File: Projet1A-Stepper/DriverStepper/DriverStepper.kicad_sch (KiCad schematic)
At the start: 26 parts, among them IC1 AS5600-ASOT, IC2 TMC2225-SA, J1 Conn_01x04_Pin, J2 173010542, U1 STM32F446RETx, U2 AZ1117IH-3.3TRG1

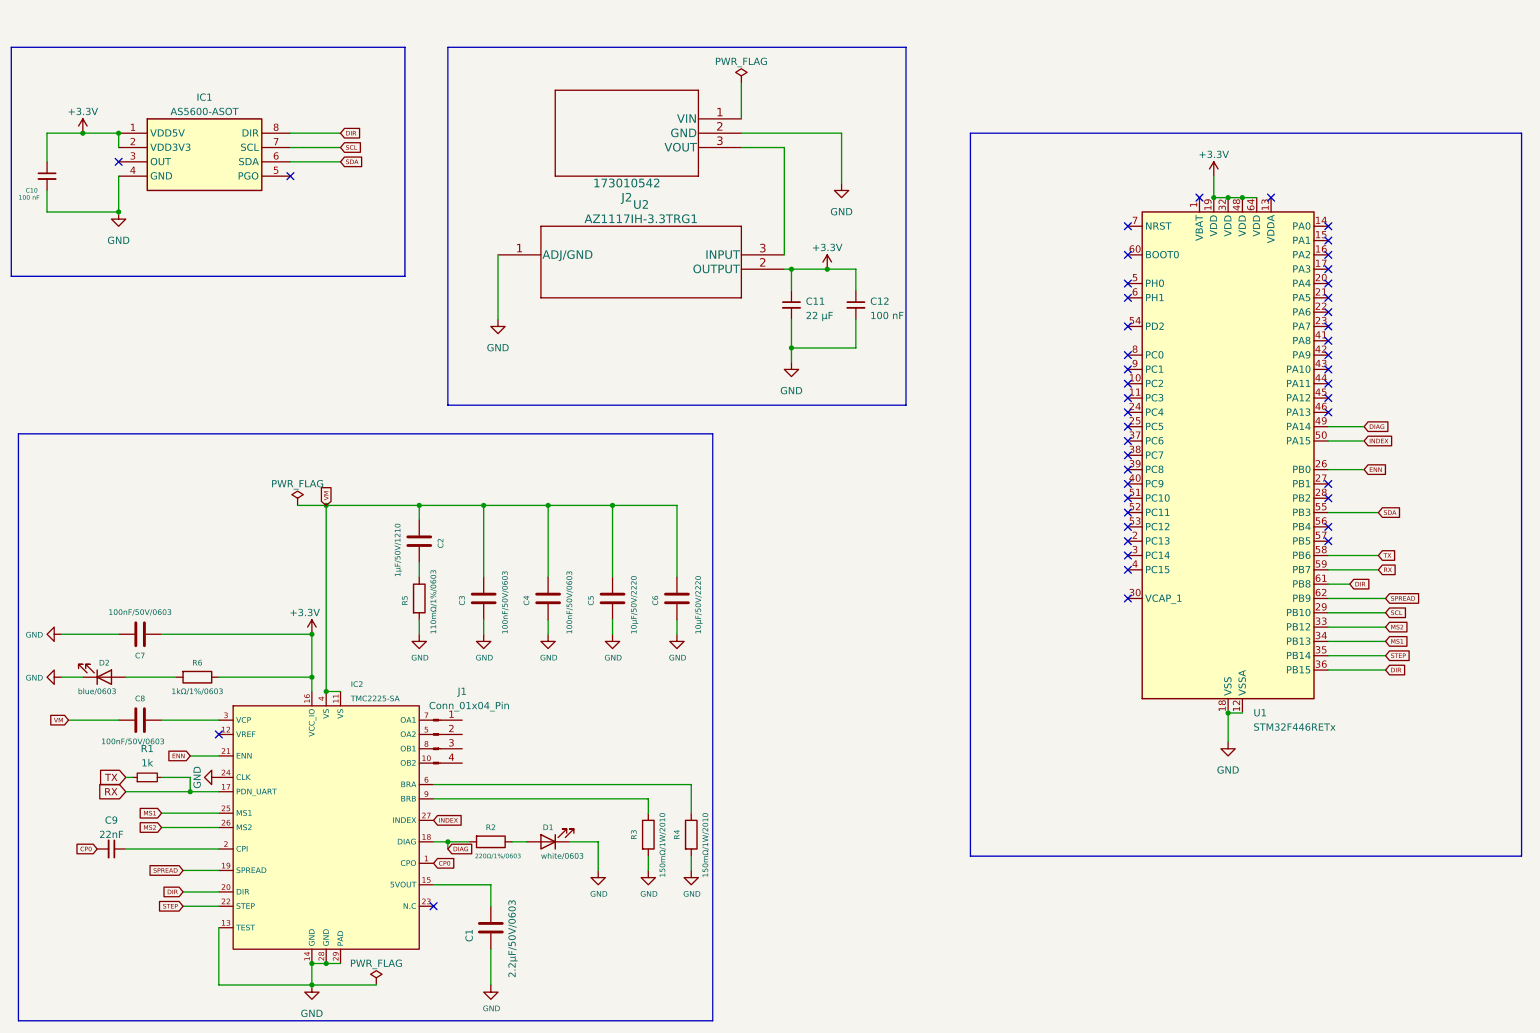
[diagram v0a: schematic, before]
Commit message: Add files via upload
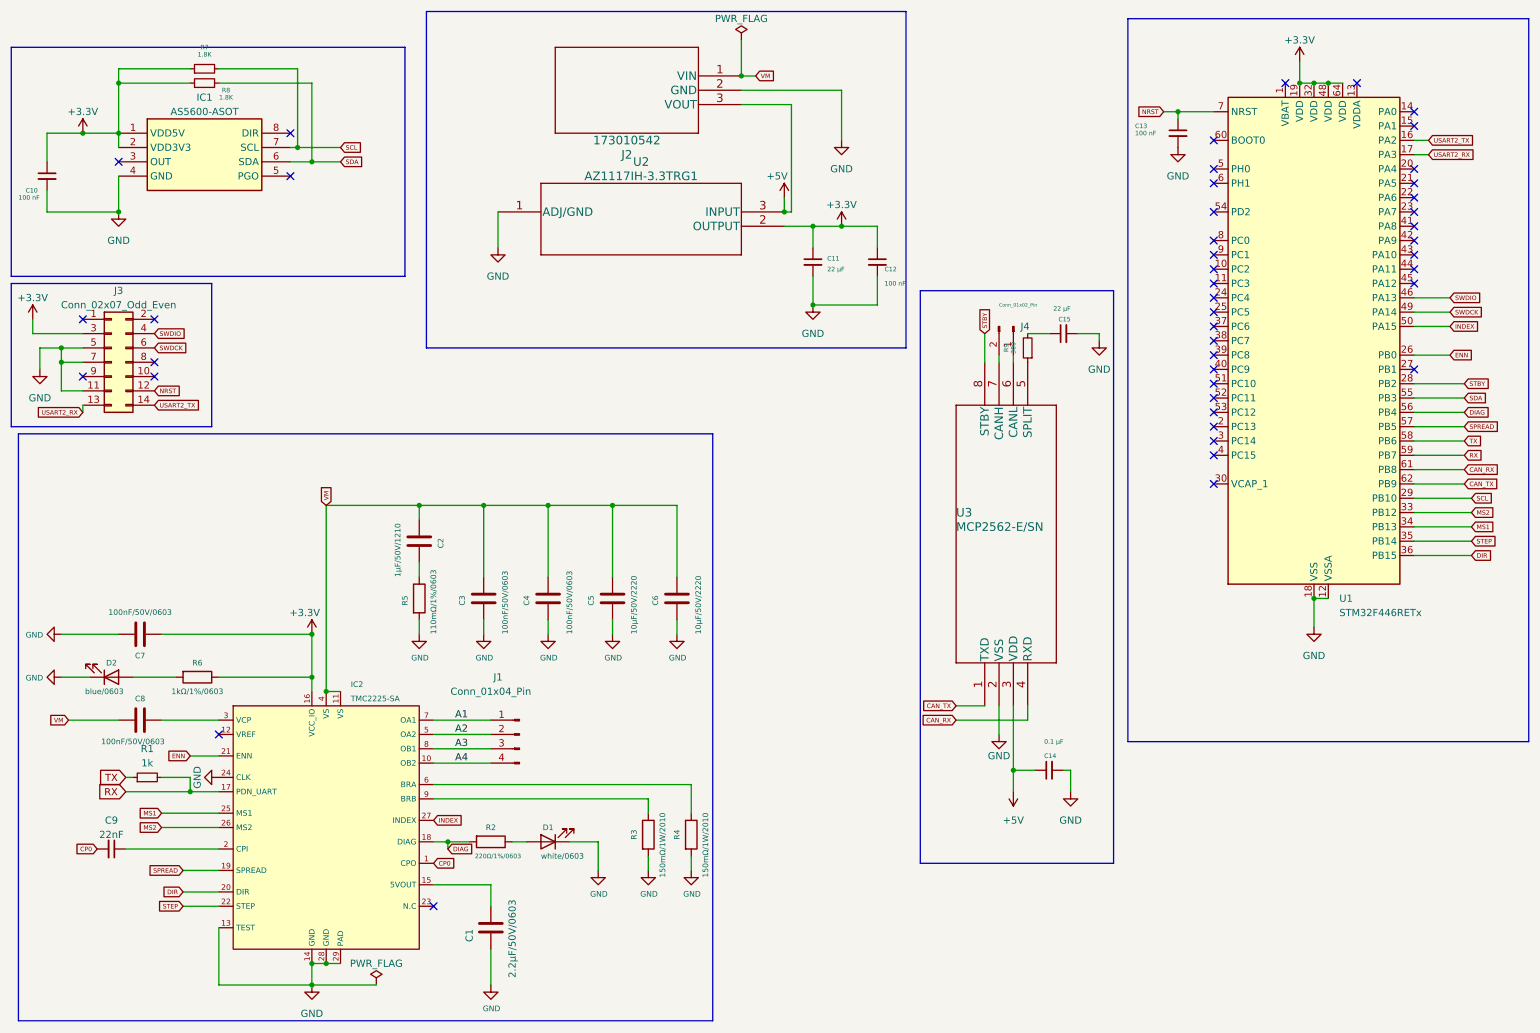
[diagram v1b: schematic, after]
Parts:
- added C13: 100 nF, symbol Device:C_Small
- added C14: 0.1 µF, symbol Device:C_Small
- added C15: 22 µF, symbol Device:C_Small
- added J3: Conn_02x07_Odd_Even, symbol Connector_Generic:Conn_02x07_Odd_Even
- added J4: Conn_01x02_Pin, symbol Connector:Conn_01x02_Pin
- added R7, R8: 1.8K, symbol Device:R_Small
- added R9: 300, symbol Device:R_Small
- added U3: MCP2562-E/SN, SOIC8-N_MC_MCH, symbol MCP2562-E/SN:MCP2562-E/SN
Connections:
- net +3.3V: now also J3.3 (Pin_3), R7.1, R8.1
- net DIAG: now also U1.56 (PB4); no longer U1.49 (PA14)
- net DIR: no longer IC1.8 (DIR), U1.61 (PB8)
- net GND: now also C13.2, C14.2, C15.2, J3.11 (Pin_11), J3.5 (Pin_5), J3.7 (Pin_7), U3.2 (VSS)
- net SCL: now also R7.2
- net SDA: now also R8.2
- net SPREAD: now also U1.57 (PB5); no longer U1.62 (PB9)
- net VM: now also J2.1 (VIN)
- net +5V: now reaches J2.3 (VOUT), U2.3 (INPUT)
- net +5V: now also C14.1, U3.3 (VDD)
- net A4: now reaches IC2.10 (OB2)
- net A4: now also J1.4 (Pin_4)
- net A2: now reaches IC2.5 (OA2)
- net A2: now also J1.2 (Pin_2)
- net A1: now reaches IC2.7 (OA1)
- net A1: now also J1.1 (Pin_1)
- net A3: now reaches IC2.8 (OB1)
- net A3: now also J1.3 (Pin_3)
- net USART2_TX: now reaches U1.16 (PA2)
- net USART2_TX: now also J3.14 (Pin_14)
- net USART2_RX: now reaches U1.17 (PA3)
- net USART2_RX: now also J3.13 (Pin_13)
- net STBY: now reaches U1.28 (PB2)
- net STBY: now also U3.8 (STBY)
- net SWDIO: now reaches U1.46 (PA13)
- net SWDIO: now also J3.4 (Pin_4)
- net NRST: now reaches U1.7 (NRST)
- net NRST: now also C13.1, J3.12 (Pin_12)
- new net: R9.1, U3.5 (SPLIT)
- new net: C15.1, R9.2
- new net: J4.1 (Pin_1), U3.6 (CANL)
- new net: J4.2 (Pin_2), U3.7 (CANH)
- new net CAN_RX: U1.61 (PB8), U3.4 (RXD)
- new net CAN_TX: U1.62 (PB9), U3.1 (TXD)
- new net SWDCK: J3.6 (Pin_6), U1.49 (PA14)
- no-connect marks 46 -> 45
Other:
- moved on the sheet: C11, C12, D2, J1, J2, U1, U2

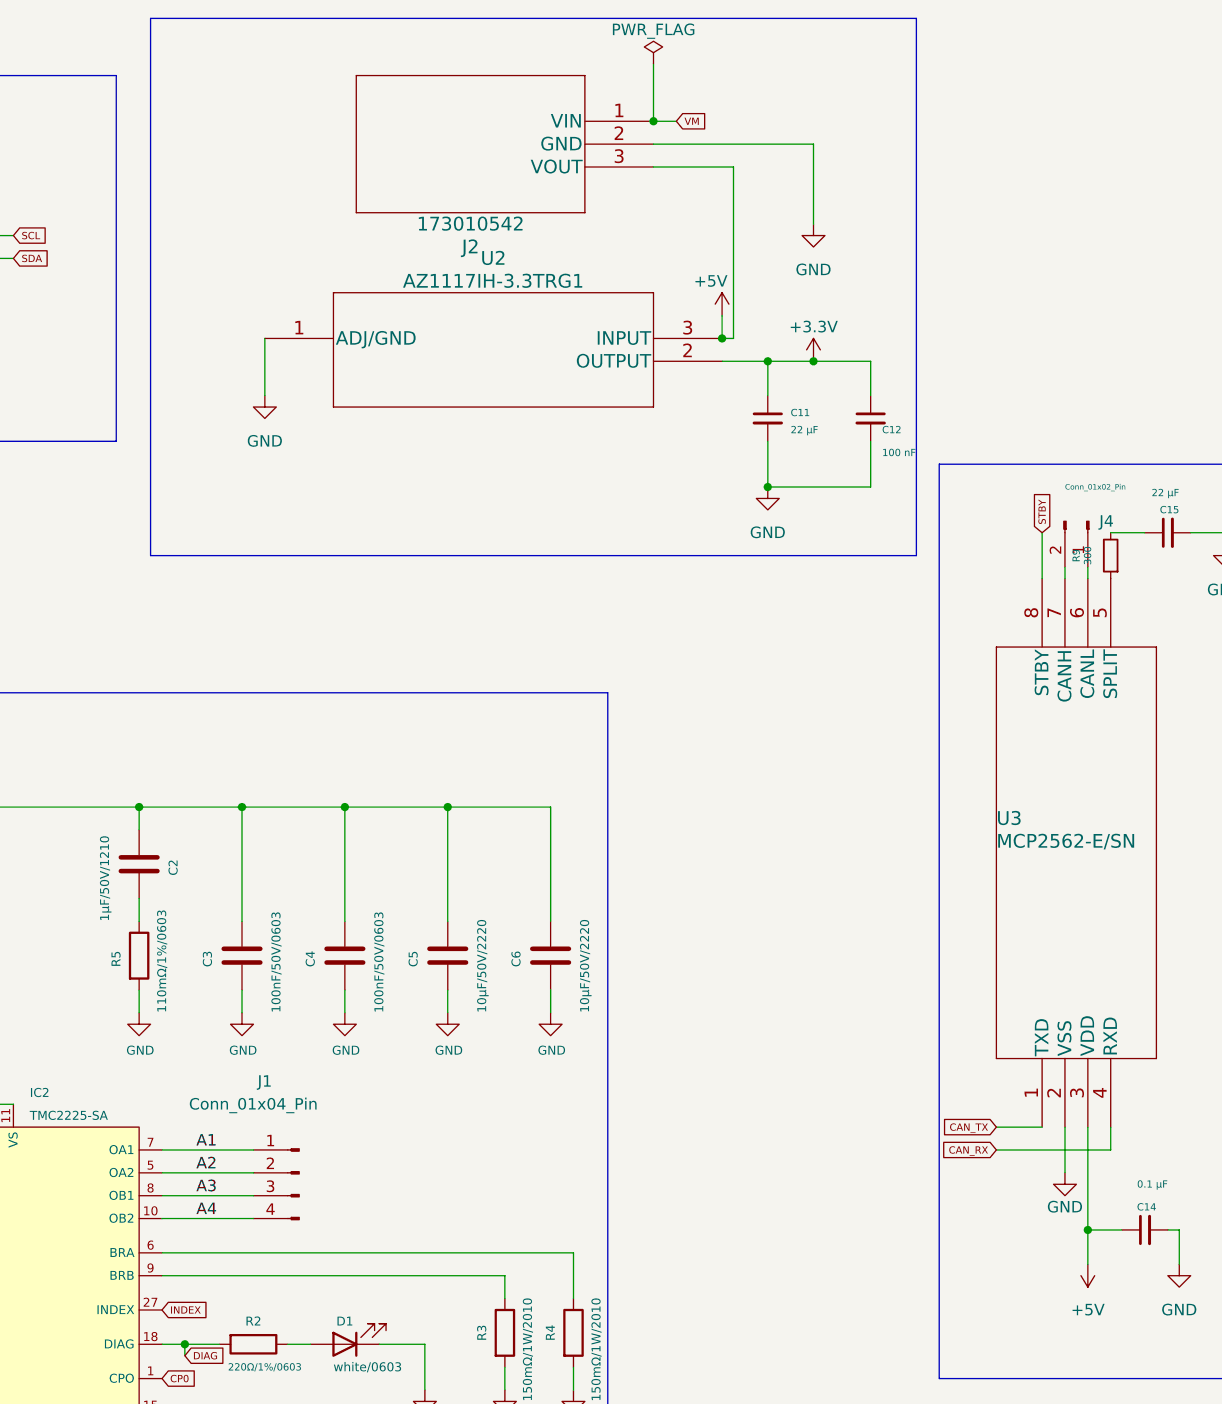
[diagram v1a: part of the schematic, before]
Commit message: Add files via upload
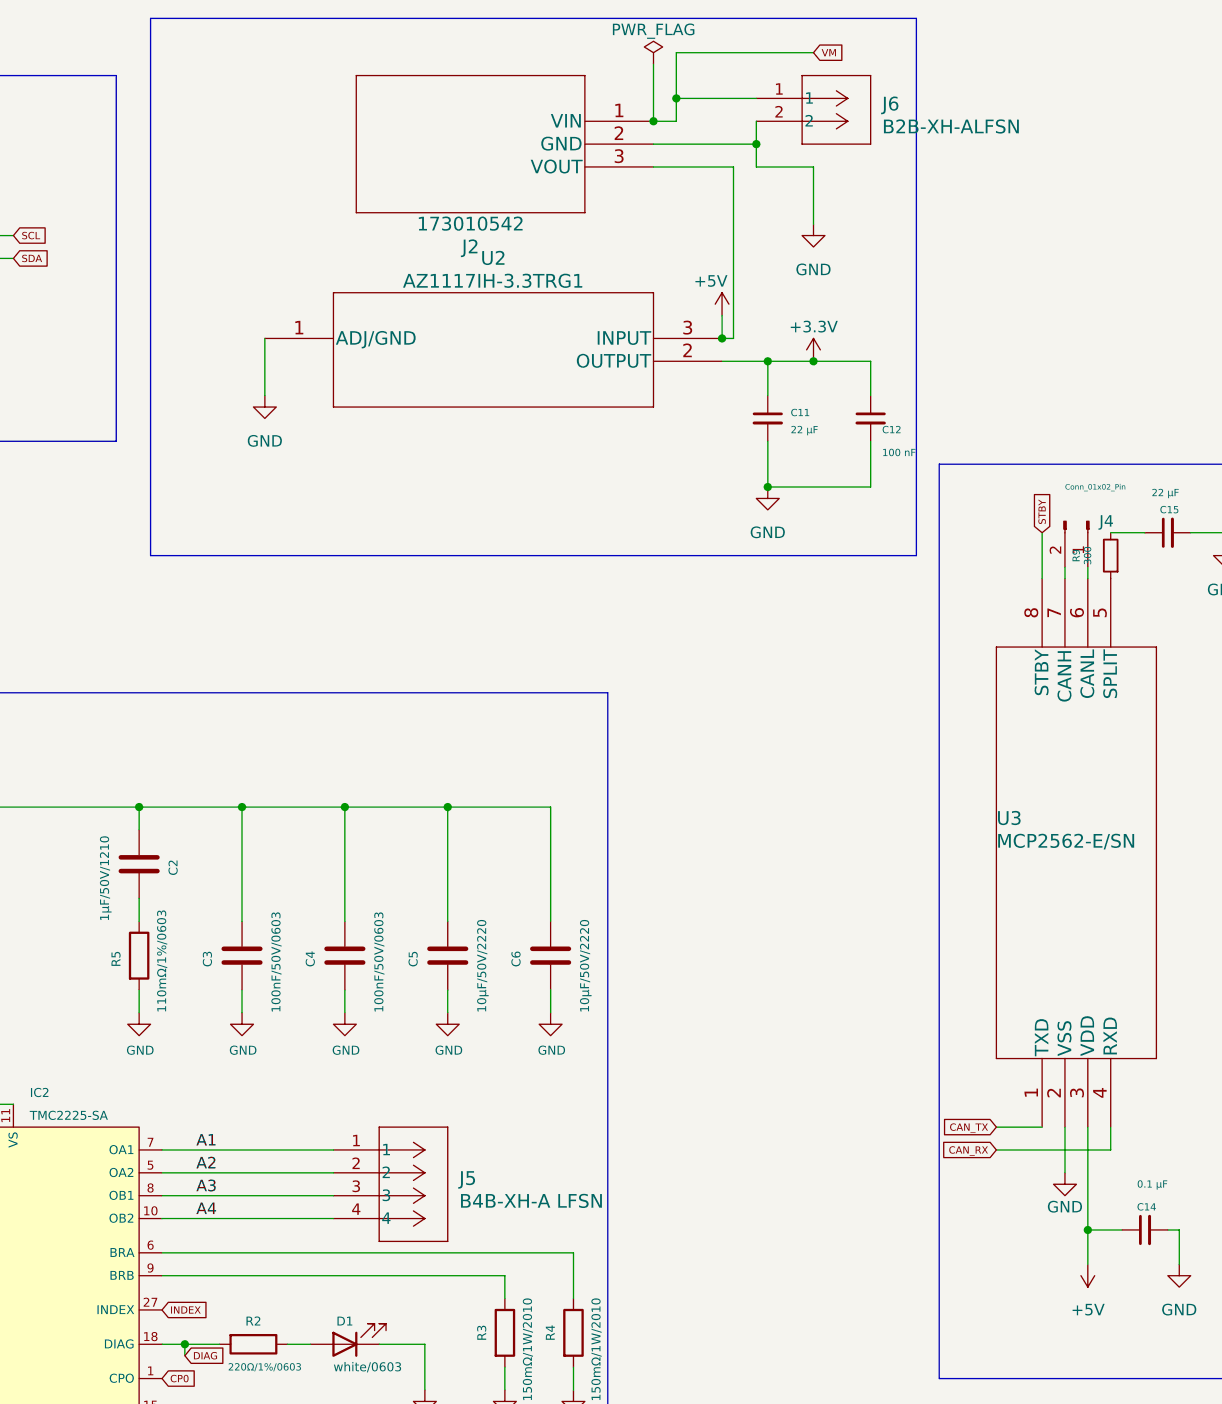
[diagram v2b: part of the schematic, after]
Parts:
- removed J1: Conn_01x04_Pin, symbol Connector:Conn_01x04_Pin
- added J5: B4B-XH-A LFSN, JST 4 PINS:CONN_B4B-XH-A LFSN_JST, symbol JST B4B-XH-A:B4B-XH-A_LFSN
- added J6: B2B-XH-ALFSN, JST 2 pins:CONN_B2B-XH-ALFSN_JST, symbol 2023-05-16_12-32-42:B2B-XH-ALFSN
- C1: footprint Capacitor_SMD:C_0603_1608Metric -> Capacitor_SMD:C_0603_1608Metric_Pad1.08x0.95mm_HandSolder
- C10, C12, C13, C14, C9, J3: footprint (none) -> Capacitor_SMD:C_0603_1608Metric_Pad1.08x0.95mm_HandSolder
- C11, C15, J4: footprint (none) -> Capacitor_SMD:C_2220_5650Metric_Pad1.97x5.40mm_HandSolder
- D1, D2: footprint LED_SMD:LED_0603_1608Metric_Castellated -> LED_SMD:LED_0603_1608Metric_Pad1.05x0.95mm_HandSolder
- IC1: footprint SOIC127P600X175-8N -> AS5600:SOIC127P600X175-8N
- IC2: footprint KiCad Lib:HTSSOP-28-1EPred_4.4x9.7mm_P0.65mm_EP3.4x9.5mm -> TMC2255:HTSSOP28_TRI
- J2: footprint CONN3_10542_WRE -> Capacitor_SMD:C_01005_0402Metric_Pad0.57x0.30mm_HandSolder
- R1, R7, R8, R9: footprint (none) -> Resistor_SMD:R_0603_1608Metric_Pad0.98x0.95mm_HandSolder
- U2: footprint SOT223_AZ1117I_6P5X3P5_DIO -> AZ1117:AZ1117IH-3.3TRG1
- U3: footprint SOIC8-N_MC_MCH -> MCP2562-E/SN:MCP2562-E&slash_SN
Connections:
- net A1: now also J5.1
- net A2: now also J5.2
- net A3: now also J5.3
- net A4: now also J5.4
- net GND: now also J6.2
- net VM: now also J6.1
